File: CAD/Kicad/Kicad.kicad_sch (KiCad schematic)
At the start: 13 parts, among them J1 USB_B_Mini, U1 AMS1117, U2 ESP8266EX, U3 FT230XS, U4 MCP3208, U5 MCP23017x-x-SS, U6 ESP32-S3

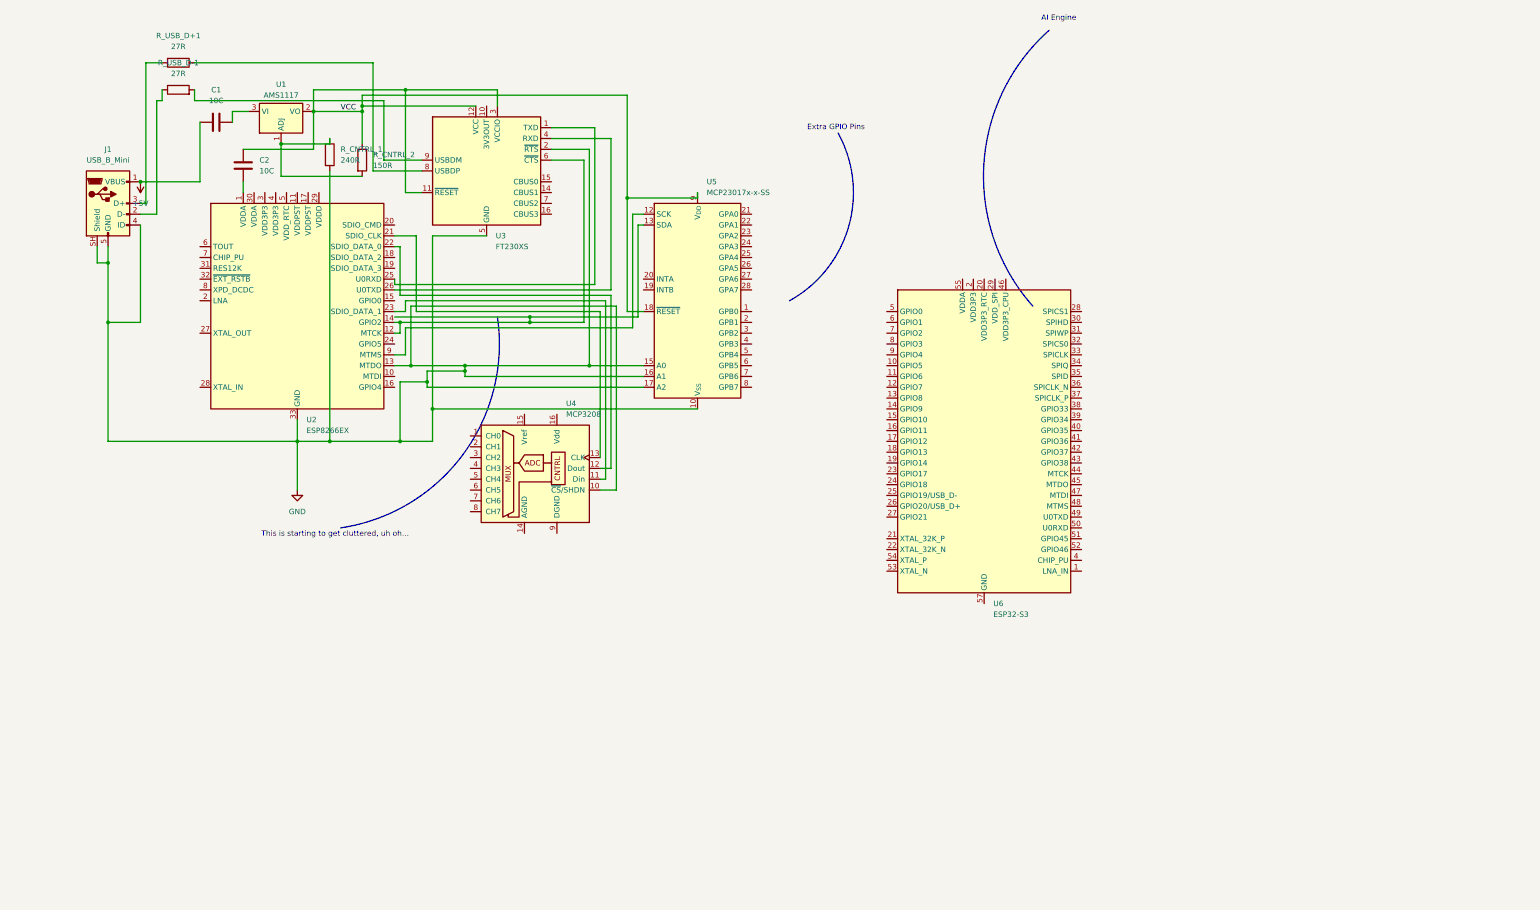
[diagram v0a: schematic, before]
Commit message: Tweaked out and redid the entire main PCB on a Tuesday Afternoon
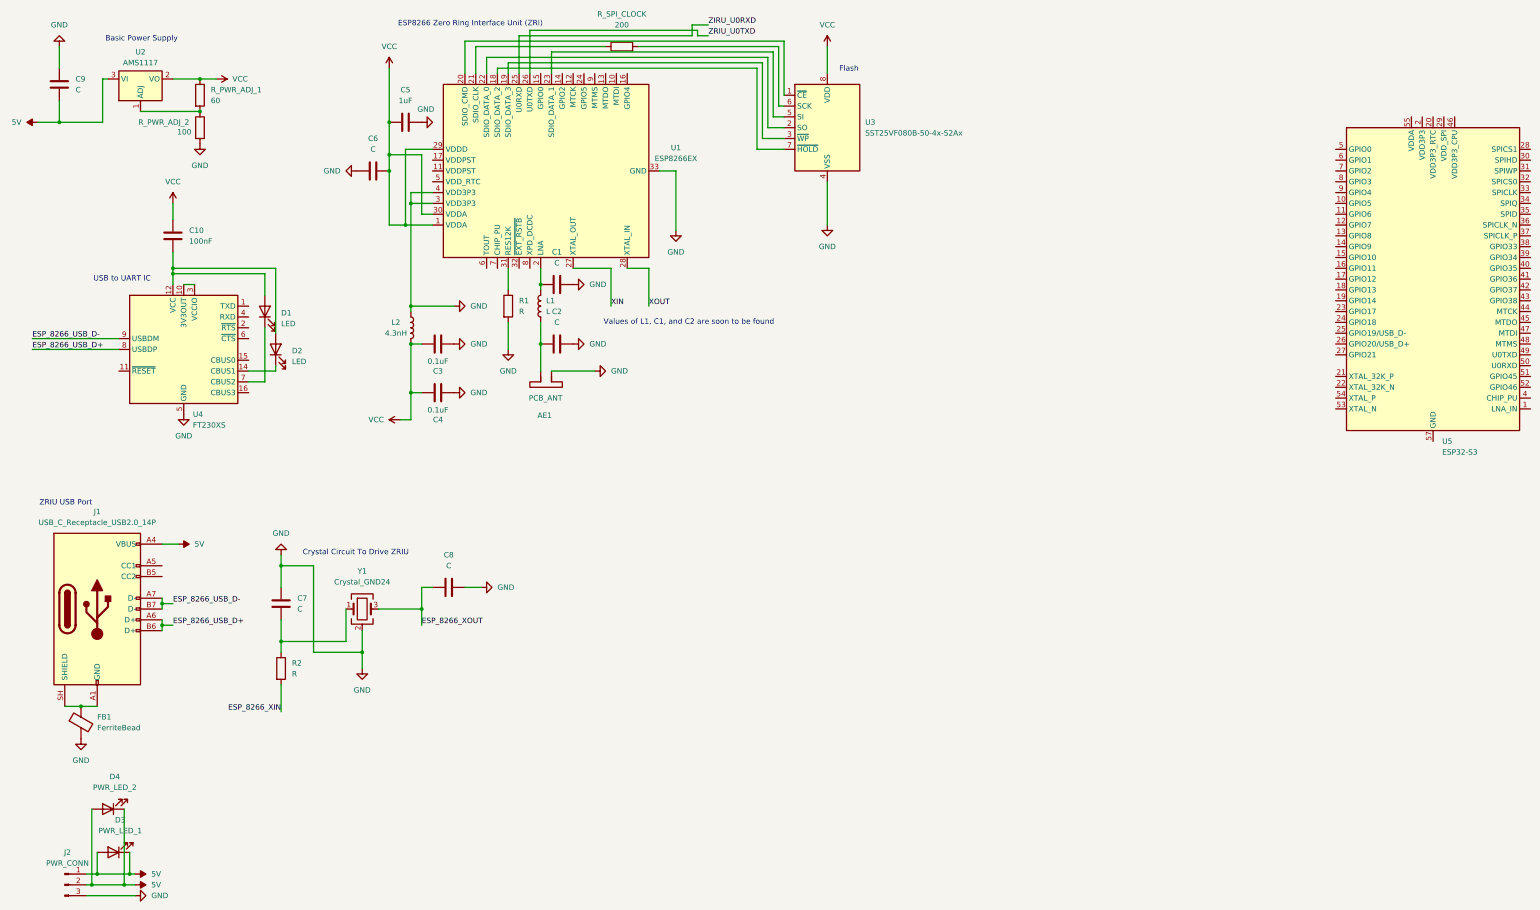
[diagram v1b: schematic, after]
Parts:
- removed J1: USB_B_Mini, symbol Connector:USB_B_Mini
- removed R_CNTRL_1: 240R, symbol Device:R
- removed R_CNTRL_2: 150R, symbol Device:R
- removed R_USB_D+1, R_USB_D-1: 27R, symbol Device:R
- removed U1: AMS1117, Package_TO_SOT_SMD:SOT-223-3_TabPin2, symbol Regulator_Linear:AMS1117
- removed U2: ESP8266EX, Package_DFN_QFN:QFN-32-1EP_5x5mm_P0.5mm_EP3.45x3.45mm, symbol MCU_Espressif:ESP8266EX
- removed U3: FT230XS, Package_SO:SSOP-16_3.9x4.9mm_P0.635mm, symbol Interface_USB:FT230XS
- removed U4: MCP3208, symbol Analog_ADC:MCP3208
- removed U5: MCP23017x-x-SS, Package_SO:SSOP-28_5.3x10.2mm_P0.65mm, symbol Interface_Expansion:MCP23017x-x-SS
- removed U6: ESP32-S3, Package_DFN_QFN:QFN-56-1EP_7x7mm_P0.4mm_EP4x4mm, symbol MCU_Espressif:ESP32-S3
- added AE1: PCB_ANT, symbol Device:Antenna_Dipole
- added C10: 100nF, symbol Device:C
- added C3, C4: 0.1uF, symbol Device:C
- added C5: 1uF, symbol Device:C
- added C6, C7, C8, C9: C, symbol Device:C
- added D1, D2: LED, symbol Device:LED
- added D3: PWR_LED_1, symbol Device:LED
- added D4: PWR_LED_2, symbol Device:LED
- added FB1: FerriteBead, symbol Device:FerriteBead
- added J1: USB_C_Receptacle_USB2.0_14P, symbol Connector:USB_C_Receptacle_USB2.0_14P
- added J2: PWR_CONN, symbol Connector:Conn_01x03_Pin
- added L1: L, symbol Device:L
- added L2: 4.3nH, symbol Device:L
- added R1, R2: R, symbol Device:R
- added R_PWR_ADJ_1: 60, symbol Device:R
- added R_PWR_ADJ_2: 100, symbol Device:R
- added R_SPI_CLOCK: 200, symbol Device:R
- added U1: ESP8266EX, Package_DFN_QFN:QFN-32-1EP_5x5mm_P0.5mm_EP3.45x3.45mm, symbol MCU_Espressif:ESP8266EX
- added U2: AMS1117, Package_TO_SOT_SMD:SOT-223-3_TabPin2, symbol Regulator_Linear:AMS1117
- added U3: SST25VF080B-50-4x-S2Ax, Package_SO:SOIC-8_5.3x5.3mm_P1.27mm, symbol Memory_Flash:SST25VF080B-50-4x-S2Ax
- added U4: FT230XS, Package_SO:SSOP-16_3.9x4.9mm_P0.635mm, symbol Interface_USB:FT230XS
- added U5: ESP32-S3, Package_DFN_QFN:QFN-56-1EP_7x7mm_P0.4mm_EP4x4mm, symbol MCU_Espressif:ESP32-S3
- added Y1: Crystal_GND24, symbol Device:Crystal_GND24
- C1, C2: value 10C -> C
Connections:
- net GND: now also C1.1, C2.1, AE1.1, C3.1, C4.1, C5.1, C6.1, C7.1, C8.2, C9.2, FB1.2, J2.3 (Pin_3), L2.1, R1.2, R_PWR_ADJ_2.2, U1.3 (VDD3P3), U1.33 (GND), U1.4 (VDD3P3), U3.4 (VSS), U4.13 (GND), U4.5 (GND), Y1.2 (G), Y1.4 (G)
- net VCC: now also C10.1, C3.2, C4.2, C5.2, C6.2, L2.2, R_PWR_ADJ_1.1, U1.1 (VDDA), U1.29 (VDDD), U1.30 (VDDA), U2.2 (VO), U3.8 (VDD); no longer C2.1
- net at C2.2: now also AE1.2, L1.1
- net +5V: no longer names the net of C1.2
- net +5V: now also L1.2, U1.2 (LNA)
- new net: FB1.1, J1.A1 (GND), J1.A12 (GND), J1.B1 (GND), J1.B12 (GND), J1.SH (SHIELD)
- new net: U4.10 (3V3OUT), U4.3 (VCCIO)
- new net: C10.2, D1.2 (A), D2.2 (A), U4.12 (VCC)
- new net: D2.1 (K), U4.14 (CBUS1)
- new net: D1.1 (K), U4.7 (CBUS2)
- new net: C7.2, R2.1, Y1.1
- new net: R_SPI_CLOCK.1, U1.21 (SDIO_CLK)
- new net: R_SPI_CLOCK.2, U3.6 (SCK)
- new net: U1.18 (SDIO_DATA_2), U3.7 (~{HOLD})
- new net: U1.19 (SDIO_DATA_3), U3.3 (~{WP})
- new net: U1.20 (SDIO_CMD), U3.1 (~{CE})
- new net: U1.22 (SDIO_DATA_0), U3.2 (SO)
- new net: U1.23 (SDIO_DATA_1), U3.5 (SI)
- new net: R1.1, U1.31 (RES12K)
- new net: U5.2 (VDD3P3), U5.3 (VDD3P3)
- new net: U5.55 (VDDA), U5.56 (VDDA)
- new net: R_PWR_ADJ_1.2, R_PWR_ADJ_2.1, U2.1 (ADJ)
- new net 5V: C9.1, D3.1 (K), D3.2 (A), D4.1 (K), D4.2 (A), J1.A4 (VBUS), J1.A9 (VBUS), J1.B4 (VBUS), J1.B9 (VBUS), J2.1 (Pin_1), J2.2 (Pin_2), U2.3 (VI)
- new net ESP_8266_USB_D+: J1.A6 (D+), J1.B6 (D+), U4.8 (USBDP)
- new net ESP_8266_USB_D-: J1.A7 (D-), J1.B7 (D-), U4.9 (USBDM)
- new net ESP_8266_XIN: R2.2
- new net ESP_8266_XOUT: C8.1, Y1.3
- new net XIN: U1.27 (XTAL_OUT)
- new net XOUT: U1.28 (XTAL_IN)
- new net ZIRU_U0RXD: U1.25 (U0RXD)
- new net ZRIU_U0TXD: U1.26 (U0TXD)
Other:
- note added: "Basic Power Supply"
- note added: "Crystal Circuit To Drive ZRIU"
- note added: "ESP8266 Zero Ring Interface Unit (ZRI)"
- note added: "Flash"
- note added: "USB to UART IC"
- note added: "Values of L1, C1, and C2 are soon to be found"
- note added: "ZRIU USB Port"
- note removed: "AI Engine"
- note removed: "Extra GPIO Pins"
- note removed: "This is starting to get cluttered, uh oh..."
- title: (none) -> Cloudboard Processing Main Unit
